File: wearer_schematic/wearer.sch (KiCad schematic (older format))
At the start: 48 parts, among them J1 Conn_01x02_Male, J2 Conn_01x06, J3 P4:5, J4 P7, J5 P14, J6 P16:18, J7 P23, Q1 AO3400A, SW1 SW_SPST, SW2 SW_Push, SW3 SW_Push, SW4 SW_Push, U1 MQ-9B, U2 SEN-11574, U3 74HC14, U4 ESP32-WROOM-32D, U5 LSM6DSLTR, U6 RFM9-LoRa-Radio

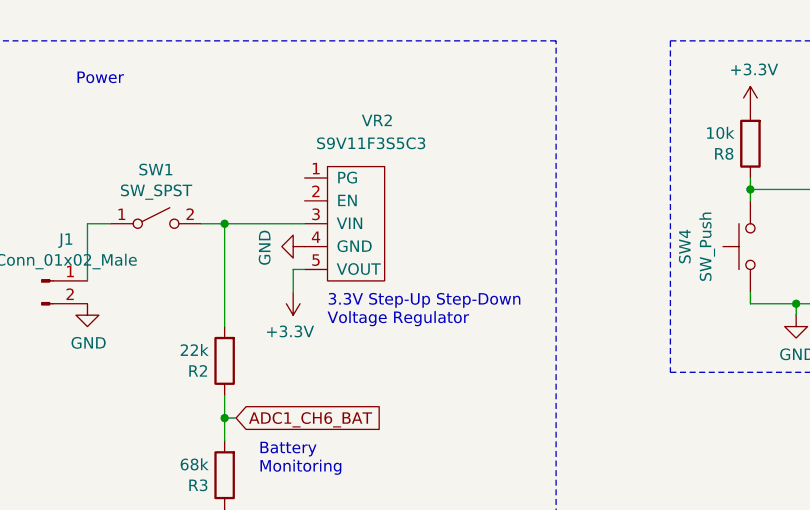
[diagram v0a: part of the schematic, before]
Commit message: before adding decoupling to power
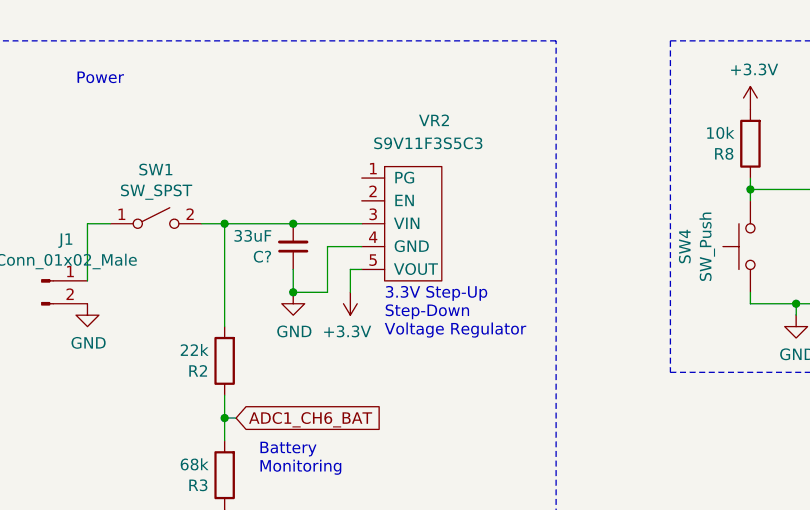
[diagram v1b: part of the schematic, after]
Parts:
- added C?: 33uF, Capacitor_SMD:C_0805_2012Metric_Pad1.15x1.40mm_HandSolder, symbol Device:C_Small
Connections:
- net GND: now also C?.1
- net at R2.2, SW1.2 (B), VR2.3 (VIN): now also C?.2
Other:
- note added: "3.3V Step-Up\nStep-Down\nVoltage Regulator"
- note removed: "3.3V Step-Up Step-Down\nVoltage Regulator"
- moved on the sheet: VR2
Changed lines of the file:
@@
 L power:GND #PWR010
 U 1 1 6219E17C
-P 2100 1550
-F 0 "#PWR010" H 2100 1300 50  0001 C CNN
-F 1 "GND" H 2105 1377 50  0000 C CNN
-F 2 "" H 2100 1550 50  0001 C CNN
-F 3 "" H 2100 1550 50  0001 C CNN
-	1    2100 1550
-	0    1    1    0
+P 2050 1750
+F 0 "#PWR010" H 2050 1500 50  0001 C CNN
+F 1 "GND" H 2055 1577 50  0000 C CNN
+F 2 "" H 2050 1750 50  0001 C CNN
+F 3 "" H 2050 1750 50  0001 C CNN
+	1    2050 1750
+	1    0    0    -1
 $EndComp
 $Comp
@@
 Text Notes 1100 850  0    50   ~ 0
 Power
-Text Notes 2200 1900 0    50   ~ 0
-3.3V Step-Up Step-Down\nVoltage Regulator
+Text Notes 2450 1950 0    50   ~ 0
+3.3V Step-Up\nStep-Down\nVoltage Regulator
 $Comp
 L Device:R R2
@@
 Wire Wire Line
 	1750 1450 1750 1900
-Wire Wire Line
-	1750 1450 2100 1450
 Text Notes 1900 2550 0    50   ~ 0
 Battery\nMonitoring
@@
 Wire Wire Line
 	1650 1450 1750 1450
-Connection ~ 1750 1450
 $Comp
 L Switch:SW_Push SW4
@@
 L Noggin:S9V11F3S5C3 VR2
 U 1 1 62215EA1
-P 2300 1450
-F 0 "VR2" V 1850 1500 50  0000 L CNN
-F 1 "S9V11F3S5C3" V 1950 1300 50  0000 L CNN
-F 2 "noggin:S9V11F3S5C3" H 2200 900 50  0001 C CNN
-F 3 "" H 2200 900 50  0001 C CNN
-	1    2300 1450
+P 2550 1450
+F 0 "VR2" V 2100 1500 50  0000 L CNN
+F 1 "S9V11F3S5C3" V 2200 1300 50  0000 L CNN
+F 2 "noggin:S9V11F3S5C3" H 2450 900 50  0001 C CNN
+F 3 "" H 2450 900 50  0001 C CNN
+	1    2550 1450
 	0    1    1    0
 $EndComp
@@
 Accelerometer
 Wire Wire Line
-	2100 1650 2050 1650
-Wire Wire Line
-	2050 1650 2050 1750
+	2350 1650 2300 1650
+Wire Wire Line
+	2300 1650 2300 1750
 $Comp
 L power:+3.3V #PWR09
 U 1 1 6219FA43
-P 2050 1750
-F 0 "#PWR09" H 2050 1600 50  0001 C CNN
-F 1 "+3.3V" H 2065 1923 50  0000 C CNN
-F 2 "" H 2050 1750 50  0001 C CNN
-F 3 "" H 2050 1750 50  0001 C CNN
-	1    2050 1750
+P 2300 1750
+F 0 "#PWR09" H 2300 1600 50  0001 C CNN
+F 1 "+3.3V" H 2315 1923 50  0000 C CNN
+F 2 "" H 2300 1750 50  0001 C CNN
+F 3 "" H 2300 1750 50  0001 C CNN
+	1    2300 1750
 	-1   0    0    1
 $EndComp
@@
 Wire Wire Line
 	9950 4000 10100 4000
+Wire Wire Line
+	1750 1450 2050 1450
+Connection ~ 1750 1450
+$Comp
+L Device:C_Small C?
+U 1 1 6232C298
+P 2050 1550
+F 0 "C?" H 2142 1596 50  0000 L CNN
+F 1 "33uF" H 2142 1505 50  0000 L CNN
+F 2 "Capacitor_SMD:C_0805_2012Metric_Pad1.15x1.40mm_HandSolder" H 2050 1550 50  0001 C CNN
+F 3 "~" H 2050 1550 50  0001 C CNN
+	1    2050 1550
+	-1   0    0    1
+$EndComp
+Connection ~ 2050 1450
+Wire Wire Line
+	2050 1450 2350 1450
+Wire Wire Line
+	2050 1650 2050 1750
+Wire Wire Line
+	2350 1550 2200 1550
+Wire Wire Line
+	2200 1550 2200 1750
+Wire Wire Line
+	2200 1750 2050 1750
+Connection ~ 2050 1750
 $EndSCHEMATC

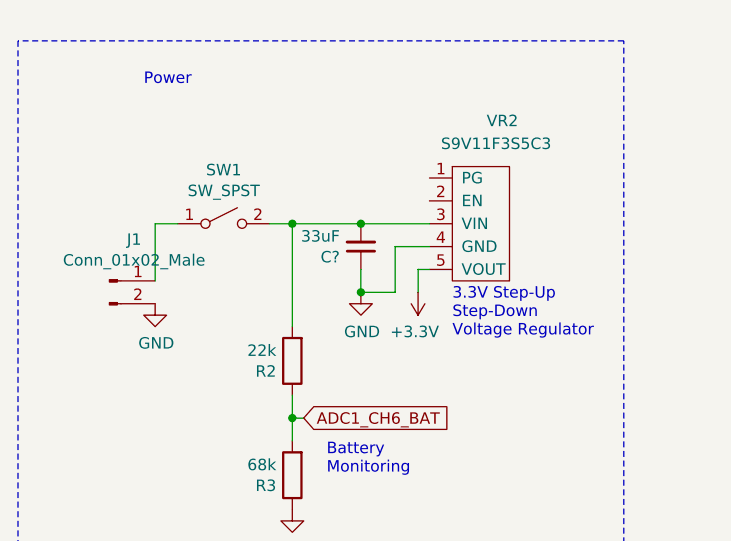
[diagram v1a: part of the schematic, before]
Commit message: pcb
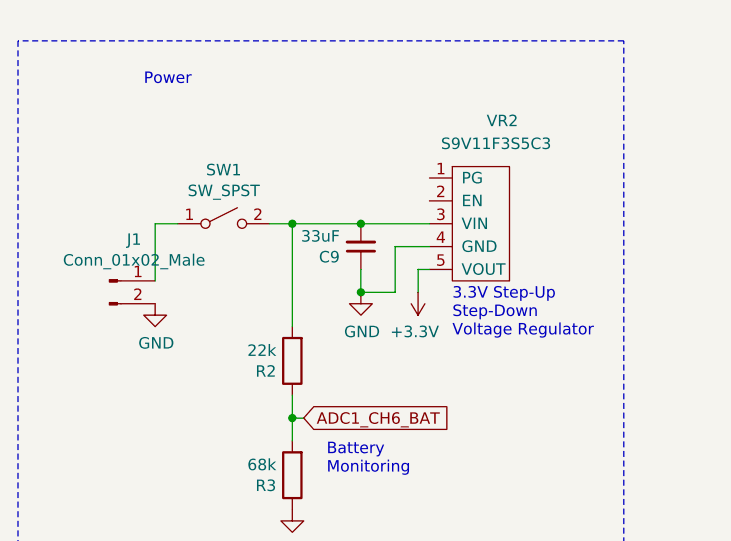
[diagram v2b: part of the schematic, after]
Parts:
- J1: footprint Connector_PinHeader_2.54mm:PinHeader_1x02_P2.54mm_Vertical -> Connector_PinHeader_2.54mm:PinHeader_1x02_P2.54mm_Horizontal
- gave numbers to parts that had none: 1
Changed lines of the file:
@@
 F 0 "J1" H 1058 1881 50  0000 C CNN
 F 1 "Conn_01x02_Male" H 1058 1790 50  0000 C CNN
-F 2 "Connector_PinHeader_2.54mm:PinHeader_1x02_P2.54mm_Vertical" H 950 1700 50  0001 C CNN
+F 2 "Connector_PinHeader_2.54mm:PinHeader_1x02_P2.54mm_Horizontal" H 950 1700 50  0001 C CNN
 F 3 "~" H 950 1700 50  0001 C CNN
 	1    950  1700
@@
 	1750 1450 2050 1450
 Connection ~ 1750 1450
-$Comp
-L Device:C_Small C?
+Connection ~ 2050 1450
+Wire Wire Line
+	2050 1450 2350 1450
+Wire Wire Line
+	2050 1650 2050 1750
+Wire Wire Line
+	2350 1550 2200 1550
+Wire Wire Line
+	2200 1550 2200 1750
+Wire Wire Line
+	2200 1750 2050 1750
+Connection ~ 2050 1750
+$Comp
+L Device:C_Small C9
 U 1 1 6232C298
 P 2050 1550
-F 0 "C?" H 2142 1596 50  0000 L CNN
+F 0 "C9" H 2142 1596 50  0000 L CNN
 F 1 "33uF" H 2142 1505 50  0000 L CNN
 F 2 "Capacitor_SMD:C_0805_2012Metric_Pad1.15x1.40mm_HandSolder" H 2050 1550 50  0001 C CNN
@@
 	-1   0    0    1
 $EndComp
-Connection ~ 2050 1450
-Wire Wire Line
-	2050 1450 2350 1450
-Wire Wire Line
-	2050 1650 2050 1750
-Wire Wire Line
-	2350 1550 2200 1550
-Wire Wire Line
-	2200 1550 2200 1750
-Wire Wire Line
-	2200 1750 2050 1750
-Connection ~ 2050 1750
 $EndSCHEMATC
